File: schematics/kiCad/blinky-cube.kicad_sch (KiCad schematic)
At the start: 25 parts, among them J1 Screw_Terminal_01x03, J2 Screw_Terminal_01x03, J3 Screw_Terminal_01x03, SW1 SW_Push, U1 Pico, U2 LM4040LP-3

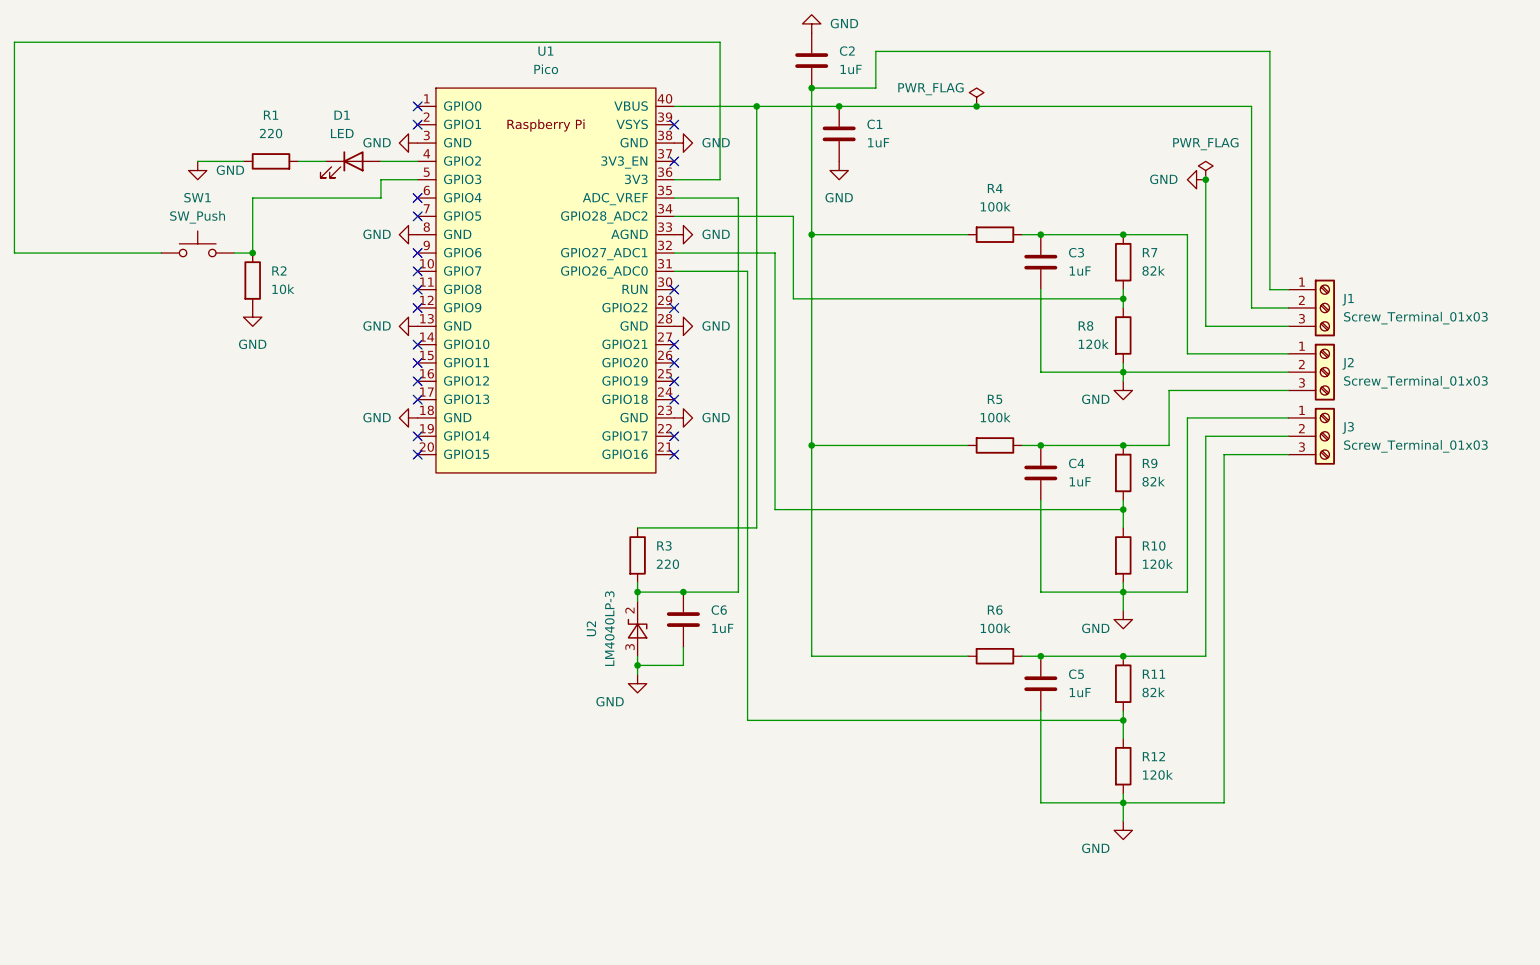
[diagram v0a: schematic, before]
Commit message: first commit
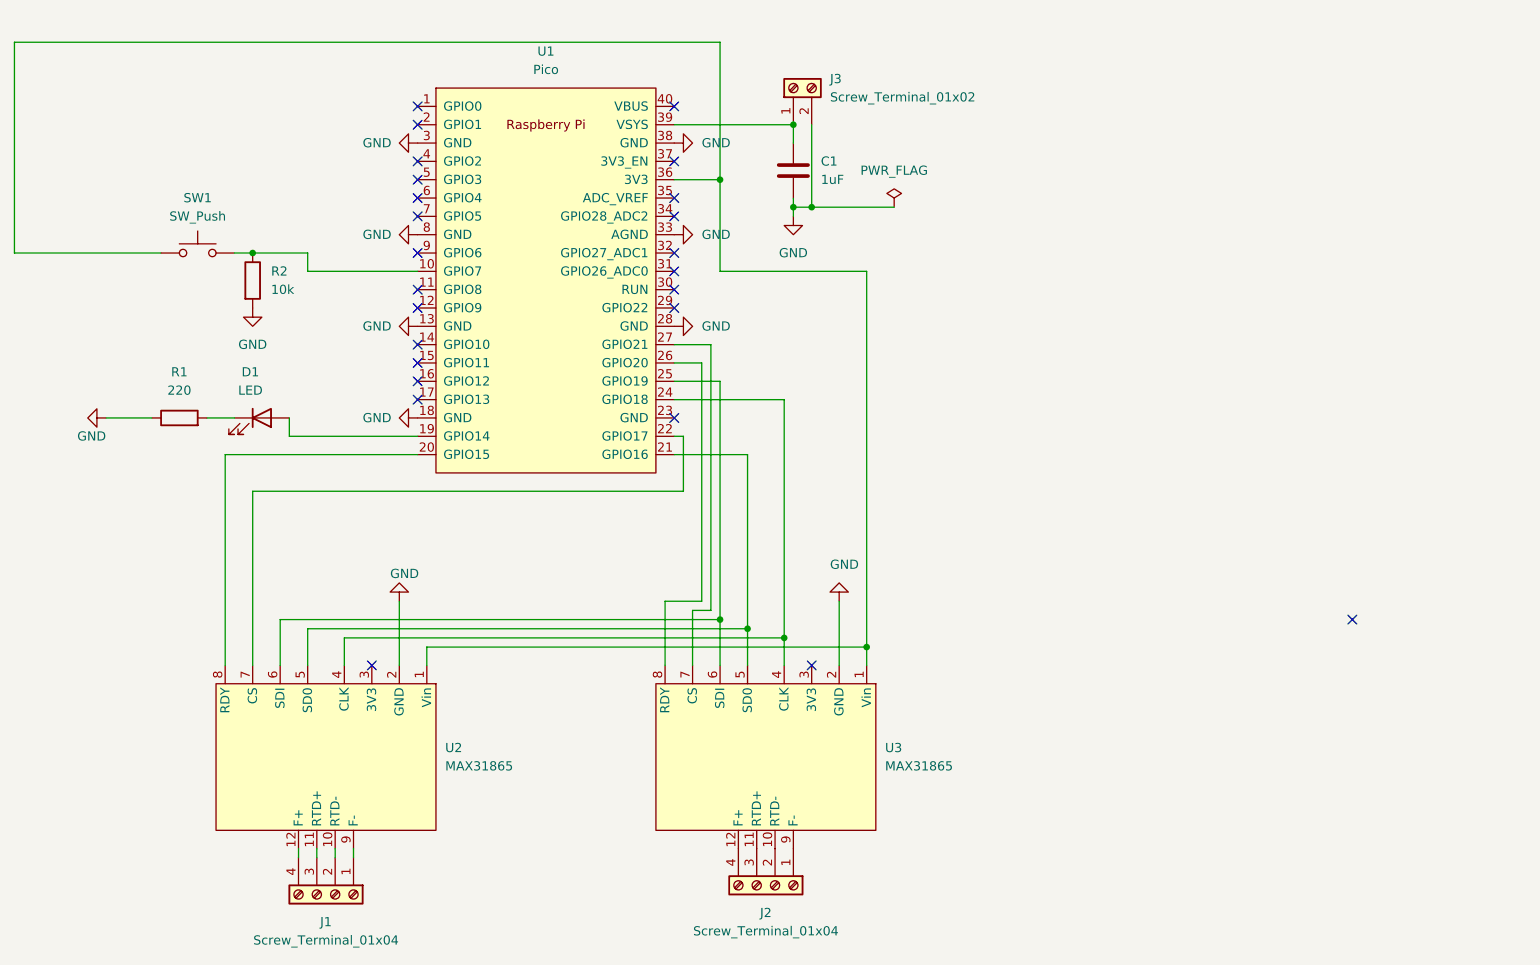
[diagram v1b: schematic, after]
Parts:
- removed C2, C3, C4, C5, C6: 1uF, Capacitor_SMD:C_1206_3216Metric_Pad1.33x1.80mm_HandSolder, symbol Device:C
- removed J1, J2, J3: Screw_Terminal_01x03, TerminalBlock:TerminalBlock_bornier-3_P5.08mm, symbol Connector:Screw_Terminal_01x03
- removed R10, R12, R8: 120k, Resistor_SMD:R_1206_3216Metric_Pad1.30x1.75mm_HandSolder, symbol Device:R
- removed R11, R7, R9: 82k, Resistor_SMD:R_1206_3216Metric_Pad1.30x1.75mm_HandSolder, symbol Device:R
- removed R3: 220, Resistor_SMD:R_1206_3216Metric_Pad1.30x1.75mm_HandSolder, symbol Device:R
- removed R4, R5, R6: 100k, Resistor_SMD:R_1206_3216Metric_Pad1.30x1.75mm_HandSolder, symbol Device:R
- removed U2: LM4040LP-3, Package_TO_SOT_THT:TO-92_Inline, symbol Reference_Voltage:LM4040LP-3
- added J1, J2: Screw_Terminal_01x04, TerminalBlock:TerminalBlock_bornier-4_P5.08mm, symbol Connector:Screw_Terminal_01x04
- added J3: Screw_Terminal_01x02, TerminalBlock:TerminalBlock_bornier-2_P5.08mm, symbol Connector:Screw_Terminal_01x02
- added U2, U3: MAX31865, MAX31865:MAX31865, symbol MAX31865:MAX31865
- C1: footprint Capacitor_SMD:C_1206_3216Metric_Pad1.33x1.80mm_HandSolder -> Capacitor_THT:C_Disc_D4.3mm_W1.9mm_P5.00mm
- R1, R2: footprint Resistor_SMD:R_1206_3216Metric_Pad1.30x1.75mm_HandSolder -> Resistor_THT:R_Axial_DIN0207_L6.3mm_D2.5mm_P7.62mm_Horizontal
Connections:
- net GND: now also J3.2 (Pin_2), U2.2 (GND), U3.2 (GND); no longer U1.23 (GND)
- net at R2.1, SW1.2: now also U1.10 (GPIO7); no longer U1.5 (GPIO3)
- net at C1.1: now also U1.39 (VSYS), J3.1 (Pin_1); no longer U1.40 (VBUS)
- net at U1.19 (GPIO14): now also D1.2 (A)
- net at U1.20 (GPIO15): now also U2.8 (RDY)
- net at U1.21 (GPIO16): now also U2.5 (SD0), U3.5 (SD0)
- net at U1.22 (GPIO17): now also U2.7 (CS)
- net at U1.24 (GPIO18): now also U2.4 (CLK), U3.4 (CLK)
- net at U1.25 (GPIO19): now also U2.6 (SDI), U3.6 (SDI)
- net at U1.26 (GPIO20): now also U3.8 (RDY)
- net at U1.27 (GPIO21): now also U3.7 (CS)
- net at SW1.1, U1.36 (3V3): now also U2.1 (Vin), U3.1 (Vin)
- net at U1.4 (GPIO2): no longer D1.2 (A)
- new net: J1.2 (Pin_2), U2.10 (RTD-)
- new net: J1.3 (Pin_3), U2.11 (RTD+)
- new net: J1.4 (Pin_4), U2.12 (F+)
- new net: J1.1 (Pin_1), U2.9 (F-)
- new net: J2.1 (Pin_1), U3.9 (F-)
- new net: J2.2 (Pin_2), U3.10 (RTD-)
- new net: J2.3 (Pin_3), U3.11 (RTD+)
- new net: J2.4 (Pin_4), U3.12 (F+)
- no-connect marks 24 -> 25
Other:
- company: (none) -> BL Monitor and Control
- title: (none) -> Blinky-RTD Cube
- moved on the sheet: C1
